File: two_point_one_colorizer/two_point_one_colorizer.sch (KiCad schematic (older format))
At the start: 33 parts, among them J1 Barrel_Jack, J2 rca, J3 mini-din4, J4 Conn_02x08_Odd_Even, J5 rca, Q1 2N3904, SW1 SPDT_slide, U1 4069, U2 LM317, U3 CD4053, Y1 3.8MHZ_Crystal, Y2 4.4MHZ_Crystal

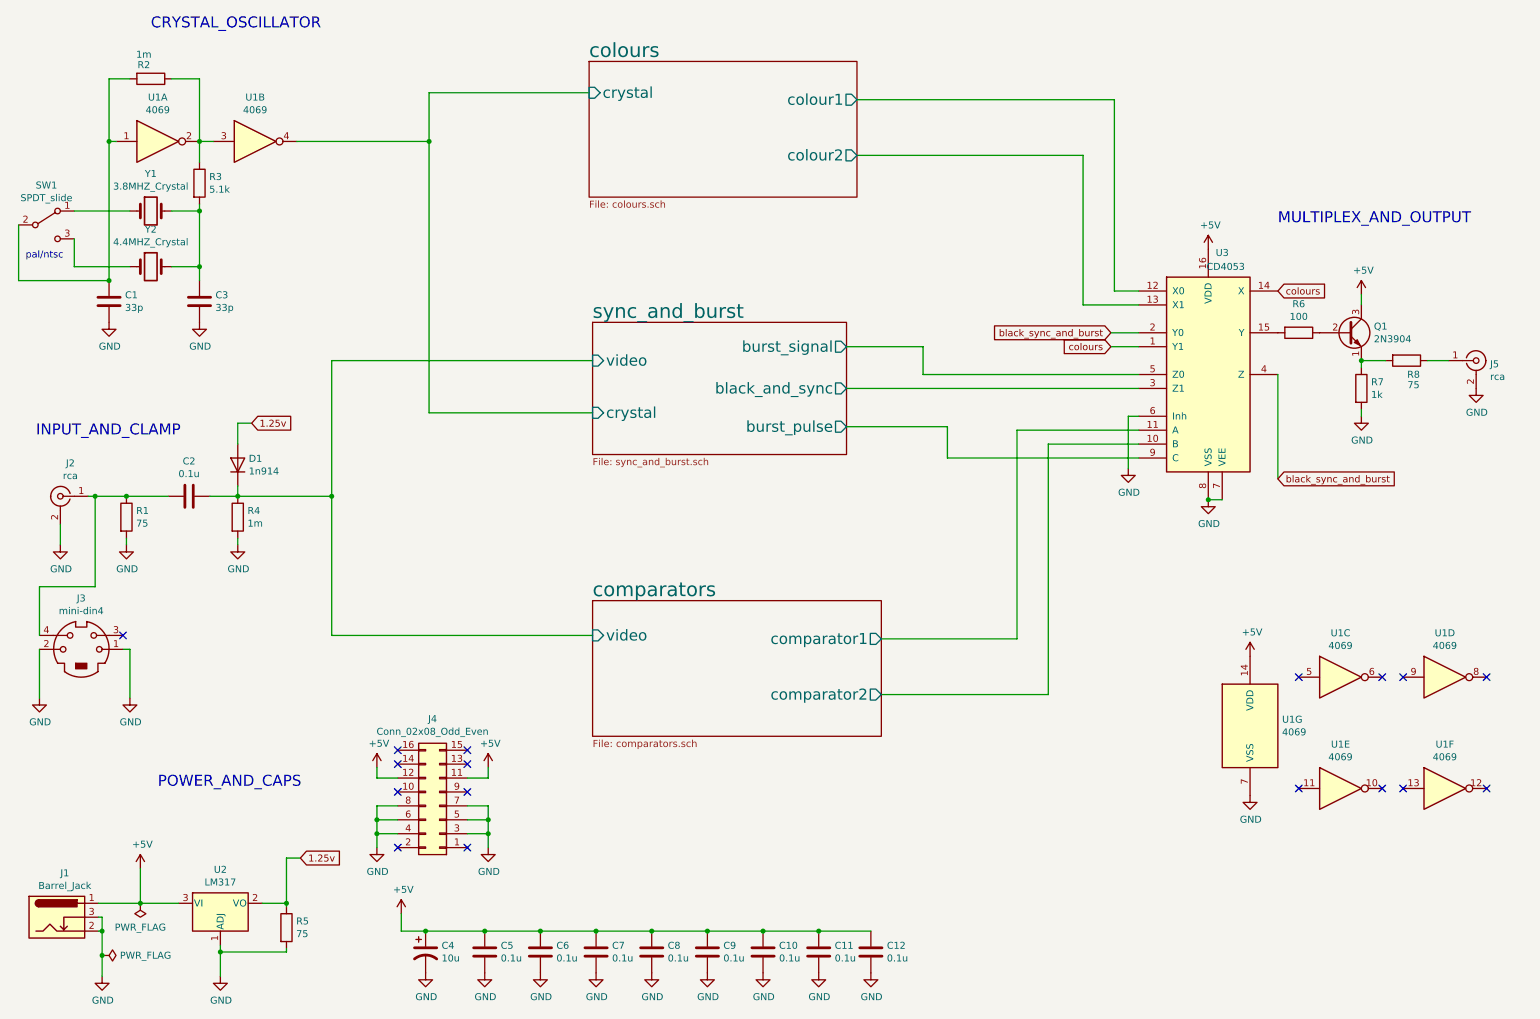
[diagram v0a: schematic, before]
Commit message: updates
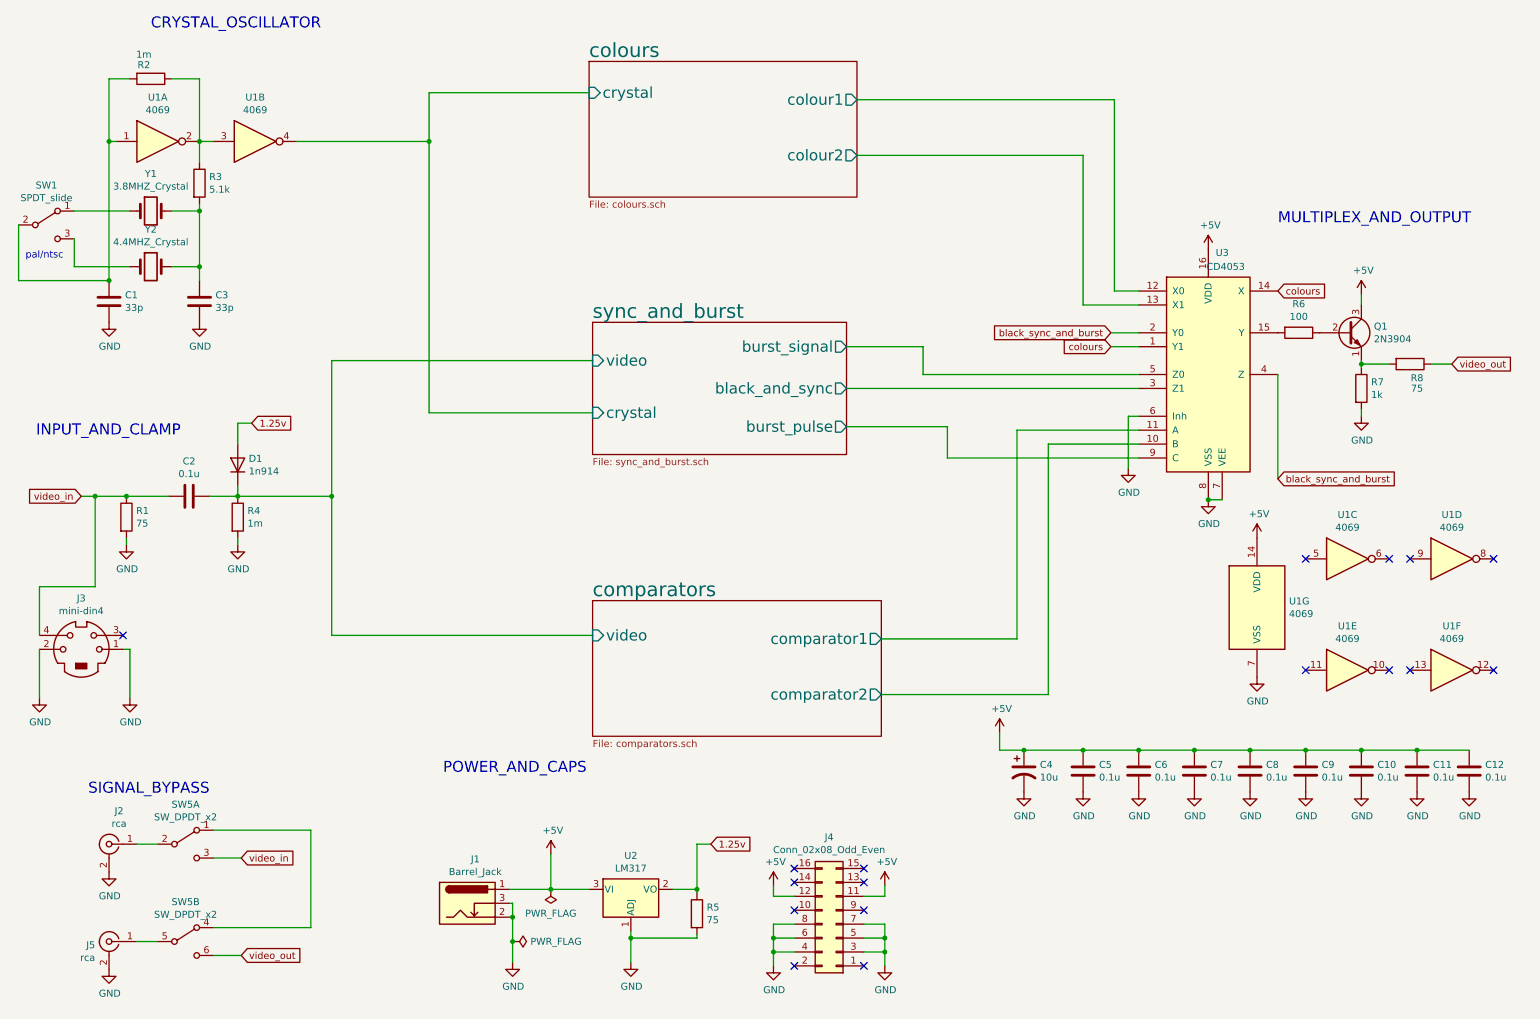
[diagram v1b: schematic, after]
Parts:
- added SW5: SW_DPDT_x2, lib_fp:dpdt_mini_toggle_switch_tayda, symbol Switch:SW_DPDT_x2
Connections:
- net video_in: now reaches C2.2, J3.4, R1.1
- net video_in: now also SW5.3 (C); no longer J2.1 (In)
- net at J5.1 (In): now also SW5.5 (B); no longer R8.1
- new net: J2.1 (In), SW5.2 (B)
- new net: SW5.1 (A), SW5.4 (A)
- new net video_out: R8.1, SW5.6 (C)
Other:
- note added: "SIGNAL_BYPASS"
- moved on the sheet: C10, C11, C12, C4, C5, C6, C7, C8, C9, J1, J2, J4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
